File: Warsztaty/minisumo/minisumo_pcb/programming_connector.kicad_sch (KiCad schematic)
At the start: 1 part

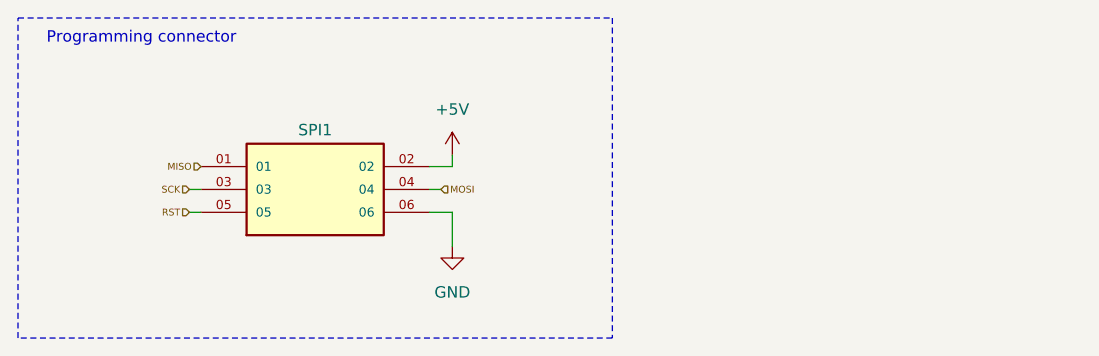
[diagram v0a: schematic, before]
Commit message: stan przed usunięciem jednego czujnika lini
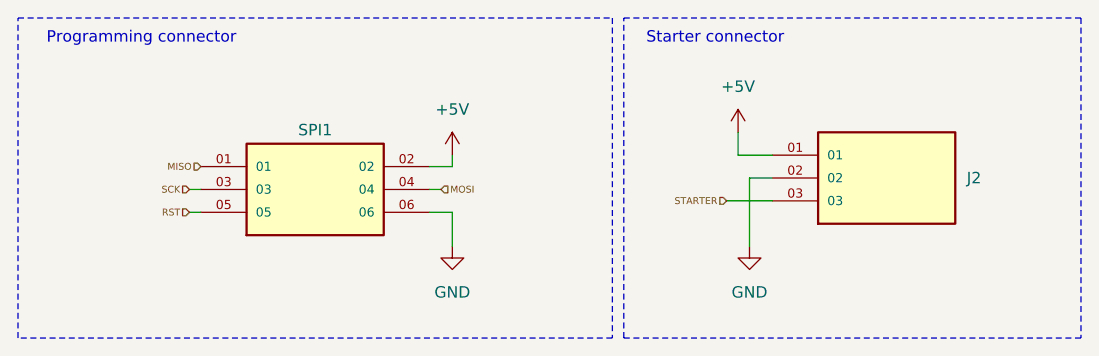
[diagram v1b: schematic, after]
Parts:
- added J2: MTSW-103-23-F-S-235, MTSW-103-23-F-S-235:SAMTEC_MTSW-103-23-F-S-235, symbol MTSW-103-23-F-S-235:MTSW-103-23-F-S-235
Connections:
- net +5V: now also J2.01
- net GND: now also J2.02
- new net STARTER: J2.03
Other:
- note added: "Starter connector"
